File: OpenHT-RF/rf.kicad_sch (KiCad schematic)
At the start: 16 parts, among them IC2 AT86RF215-ZU, IC3 RFSW8008TR7, J6 Conn_Coaxial, X1 26 MHz

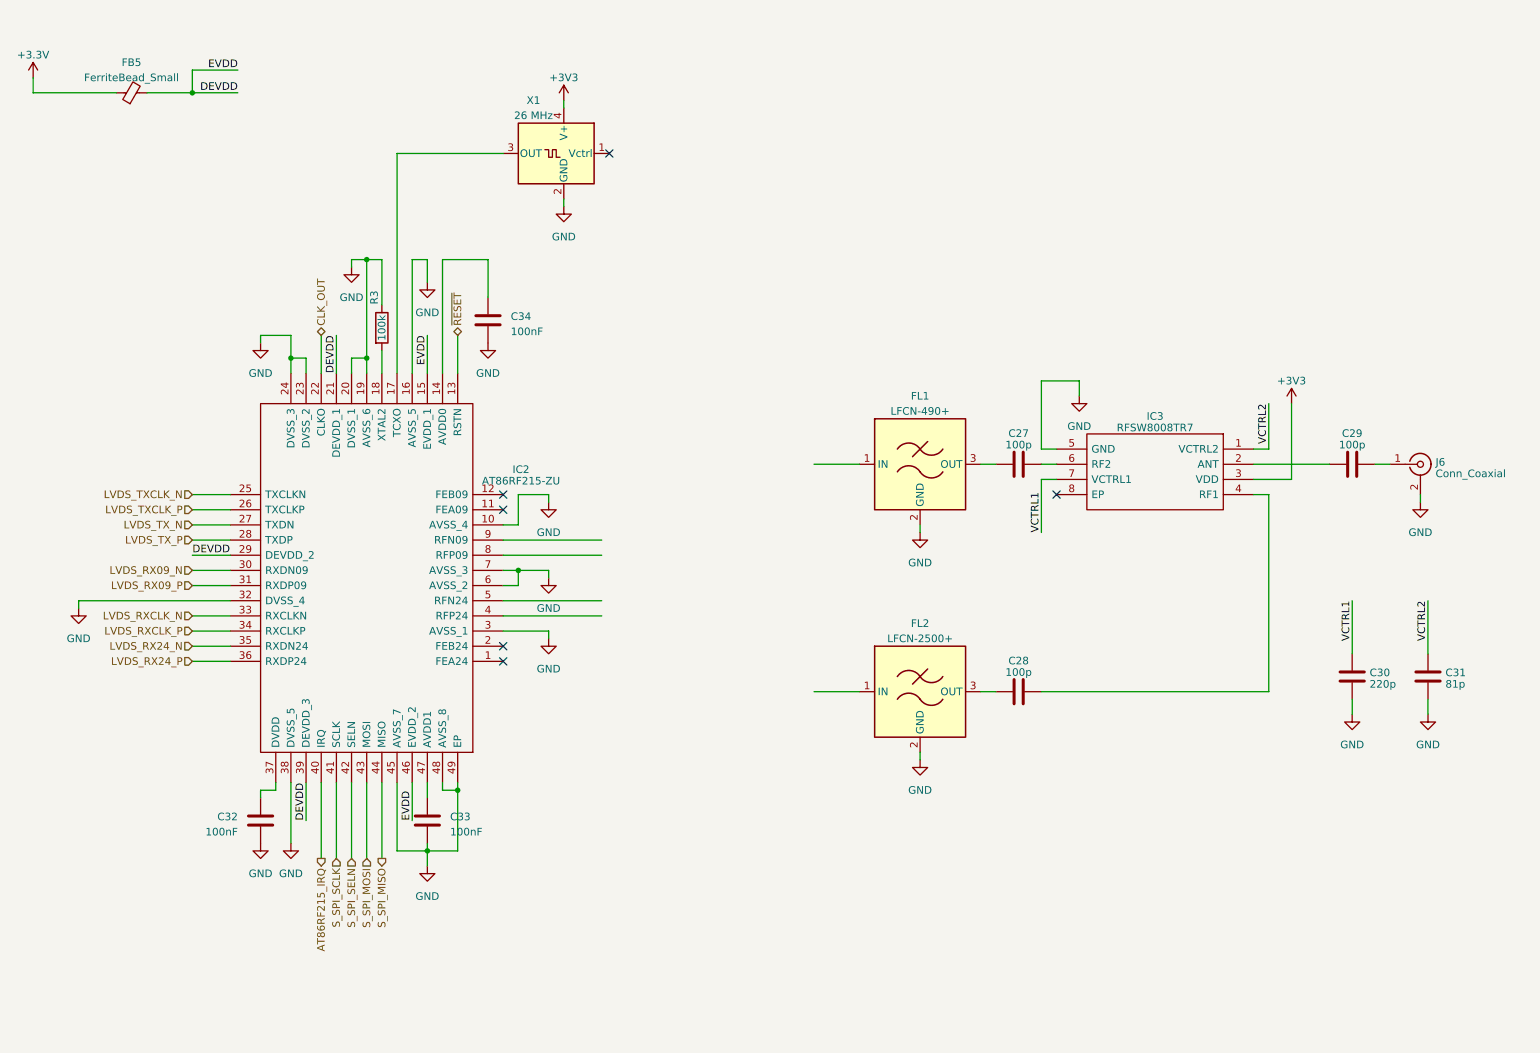
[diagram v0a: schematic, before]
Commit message: Updated RF schematic
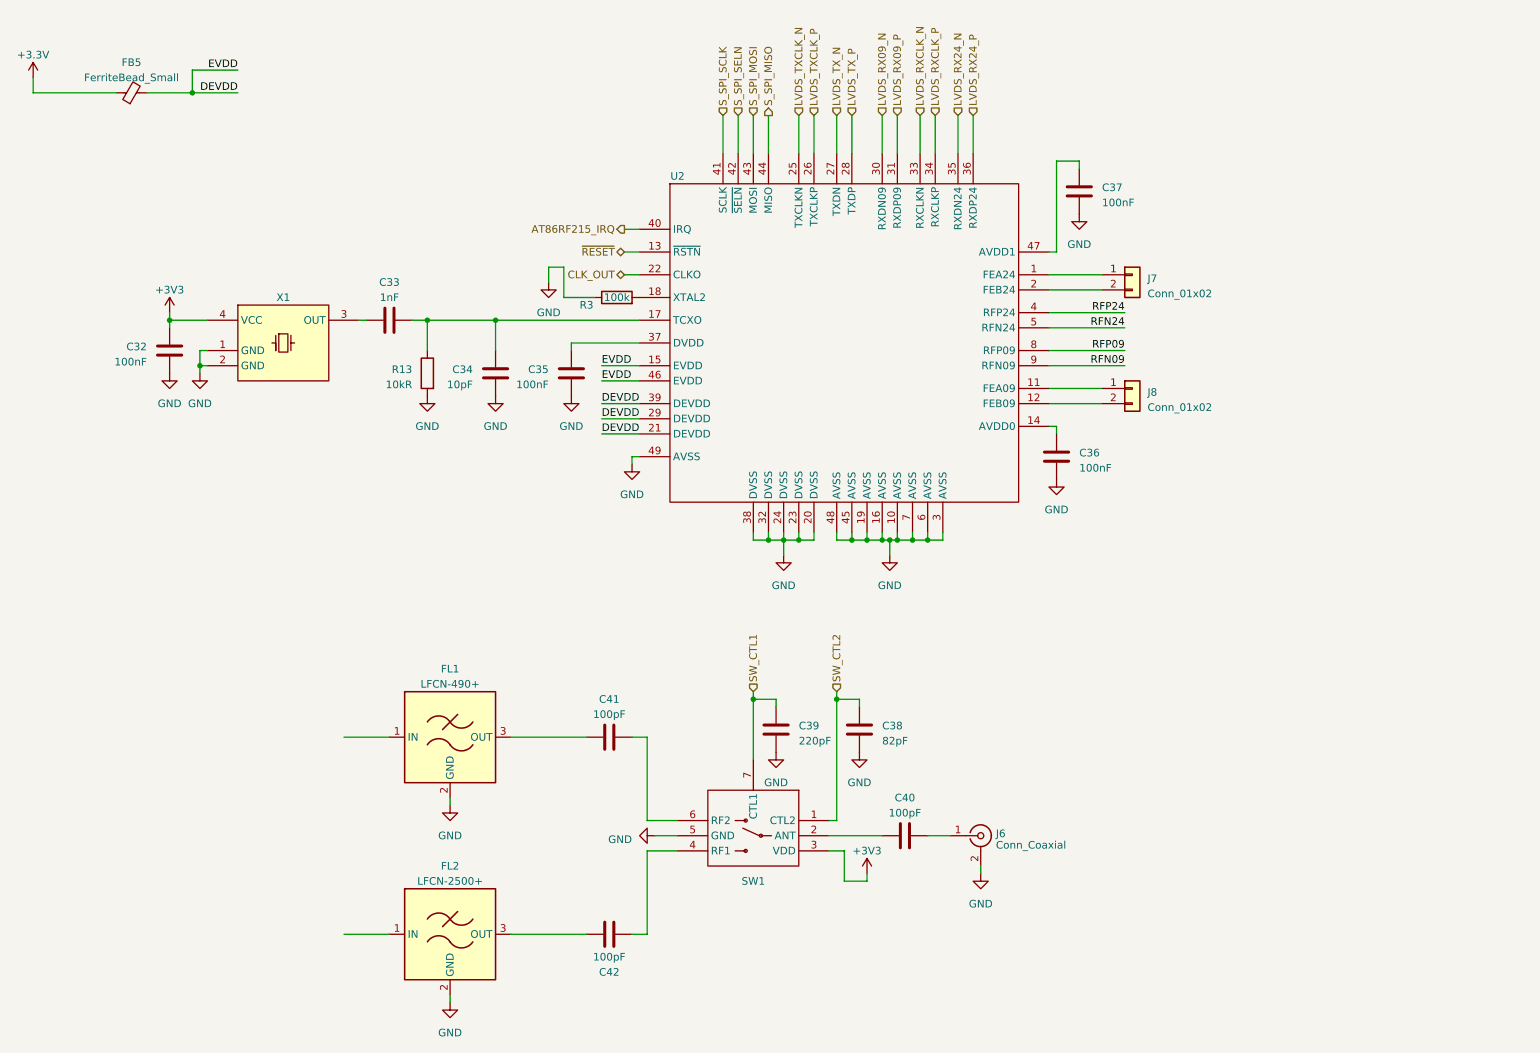
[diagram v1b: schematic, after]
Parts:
- removed C27, C28, C29: 100p, symbol Device:C
- removed C30: 220p, symbol Device:C
- removed C31: 81p, symbol Device:C
- removed IC2: AT86RF215-ZU, QFN50P700X700X90-49N-D, symbol AT86RF215-ZU:AT86RF215-ZU
- removed IC3: RFSW8008TR7, RFSW8008TR7, symbol RFSW8008TR7:RFSW8008TR7
- removed X1: 26 MHz, symbol Oscillator:DFA-S2
- added C35, C36, C37: 100nF, symbol Device:C
- added C38: 82pF, symbol Device:C
- added C39: 220pF, symbol Device:C
- added C40, C41, C42: 100pF, symbol Device:C
- added J7, J8: Conn_01x02, symbol Connector_Generic:Conn_01x02
- added R13: 10kR, symbol Device:R
- added SW1: ~, M17_misc_active:RFSW8008, symbol M17_RF:RFSW8008
- added U2: ~, M17_QFN:VQFN-48-1EP_7x7mm_P0.5mm_EP5.6x5.6mm, symbol M17_RF:AT86RF215
- added X1: ~, M17_misc_active:ECS-TXO-20CSMV, symbol M17_misc_active:ECS-TXO-20CSMV
- C33: value 100nF -> 1nF
- C34: value 100nF -> 10pF
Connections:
- net +3V3: now also C32.1, SW1.3 (VDD), X1.4 (VCC)
- net AT86RF215_IRQ: now also U2.40 (IRQ)
- net CLK_OUT: now also U2.22 (CLKO)
- net DEVDD: now also U2.15 (EVDD), U2.21 (DEVDD), U2.29 (DEVDD), U2.39 (DEVDD), U2.46 (EVDD)
- net GND: now also C35.2, C36.2, C37.2, C38.2, C39.2, R13.2, SW1.5 (GND), U2.10 (AVSS), U2.16 (AVSS), U2.19 (AVSS), U2.20 (DVSS), U2.23 (DVSS), U2.24 (DVSS), U2.3 (AVSS), U2.32 (DVSS), U2.38 (DVSS), U2.45 (AVSS), U2.48 (AVSS), U2.49 (AVSS), U2.6 (AVSS), U2.7 (AVSS), X1.1 (GND), X1.2 (GND); no longer C33.2
- net LVDS_RX09_N: now also U2.30 (RXDN09)
- net LVDS_RX09_P: now also U2.31 (RXDP09)
- net LVDS_RX24_N: now also U2.35 (RXDN24)
- net LVDS_RX24_P: now also U2.36 (RXDP24)
- net LVDS_RXCLK_N: now also U2.33 (RXCLKN)
- net LVDS_RXCLK_P: now also U2.34 (RXCLKP)
- net LVDS_TXCLK_N: now also U2.25 (TXCLKN)
- net LVDS_TXCLK_P: now also U2.26 (TXCLKP)
- net LVDS_TX_N: now also U2.27 (TXDN)
- net LVDS_TX_P: now also U2.28 (TXDP)
- net S_SPI_MISO: now also U2.44 (MISO)
- net S_SPI_MOSI: now also U2.43 (MOSI)
- net S_SPI_SCLK: now also U2.41 (SCLK)
- net S_SPI_SELN: now also U2.42 (~{SELN})
- net ~{RESET}: now also U2.13 (~{RSTN})
- net at C34.1: now also C33.2, R13.1, U2.17 (TCXO)
- net at FL1.3 (OUT): now also C41.1
- net at R3.2: now also U2.18 (XTAL2)
- net at FL2.3 (OUT): now also C42.1
- net at J6.1 (In): now also C40.2
- net at C33.1: now also X1.3 (OUT)
- new net: J7.1 (Pin_1), U2.1 (FEA24)
- new net: J8.1 (Pin_1), U2.11 (FEA09)
- new net: J8.2 (Pin_2), U2.12 (FEB09)
- new net: C36.1, U2.14 (AVDD0)
- new net: J7.2 (Pin_2), U2.2 (FEB24)
- new net: C35.1, U2.37 (DVDD)
- new net: C37.1, U2.47 (AVDD1)
- new net: C42.2, SW1.4 (RF1)
- new net: C41.2, SW1.6 (RF2)
- new net: C40.1, SW1.2 (ANT)
- new net RFN09: U2.9 (RFN09)
- new net RFN24: U2.5 (RFN24)
- new net RFP09: U2.8 (RFP09)
- new net RFP24: U2.4 (RFP24)
- new net SW_CTL1: C39.1, SW1.7 (CTL1)
- new net SW_CTL2: C38.1, SW1.1 (CTL2)
- no-connect marks 6 -> 0
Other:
- moved on the sheet: FL1, FL2
